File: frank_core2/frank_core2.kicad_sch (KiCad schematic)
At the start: 7 parts

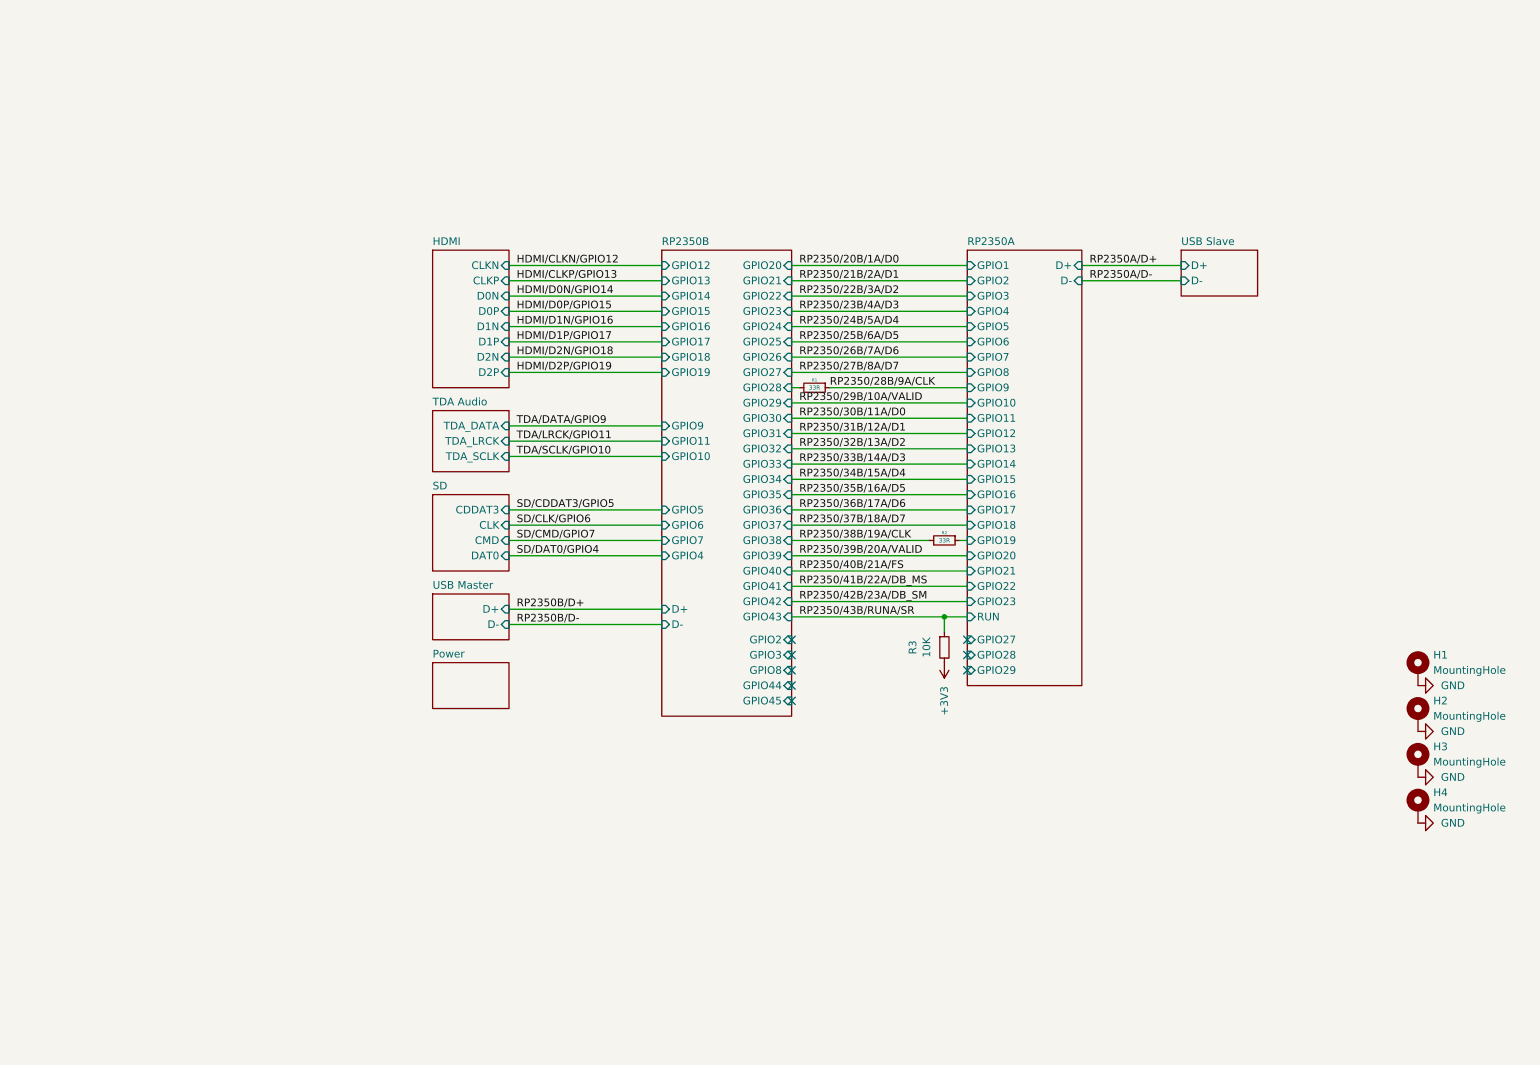
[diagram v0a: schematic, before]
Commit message: Boards WIP
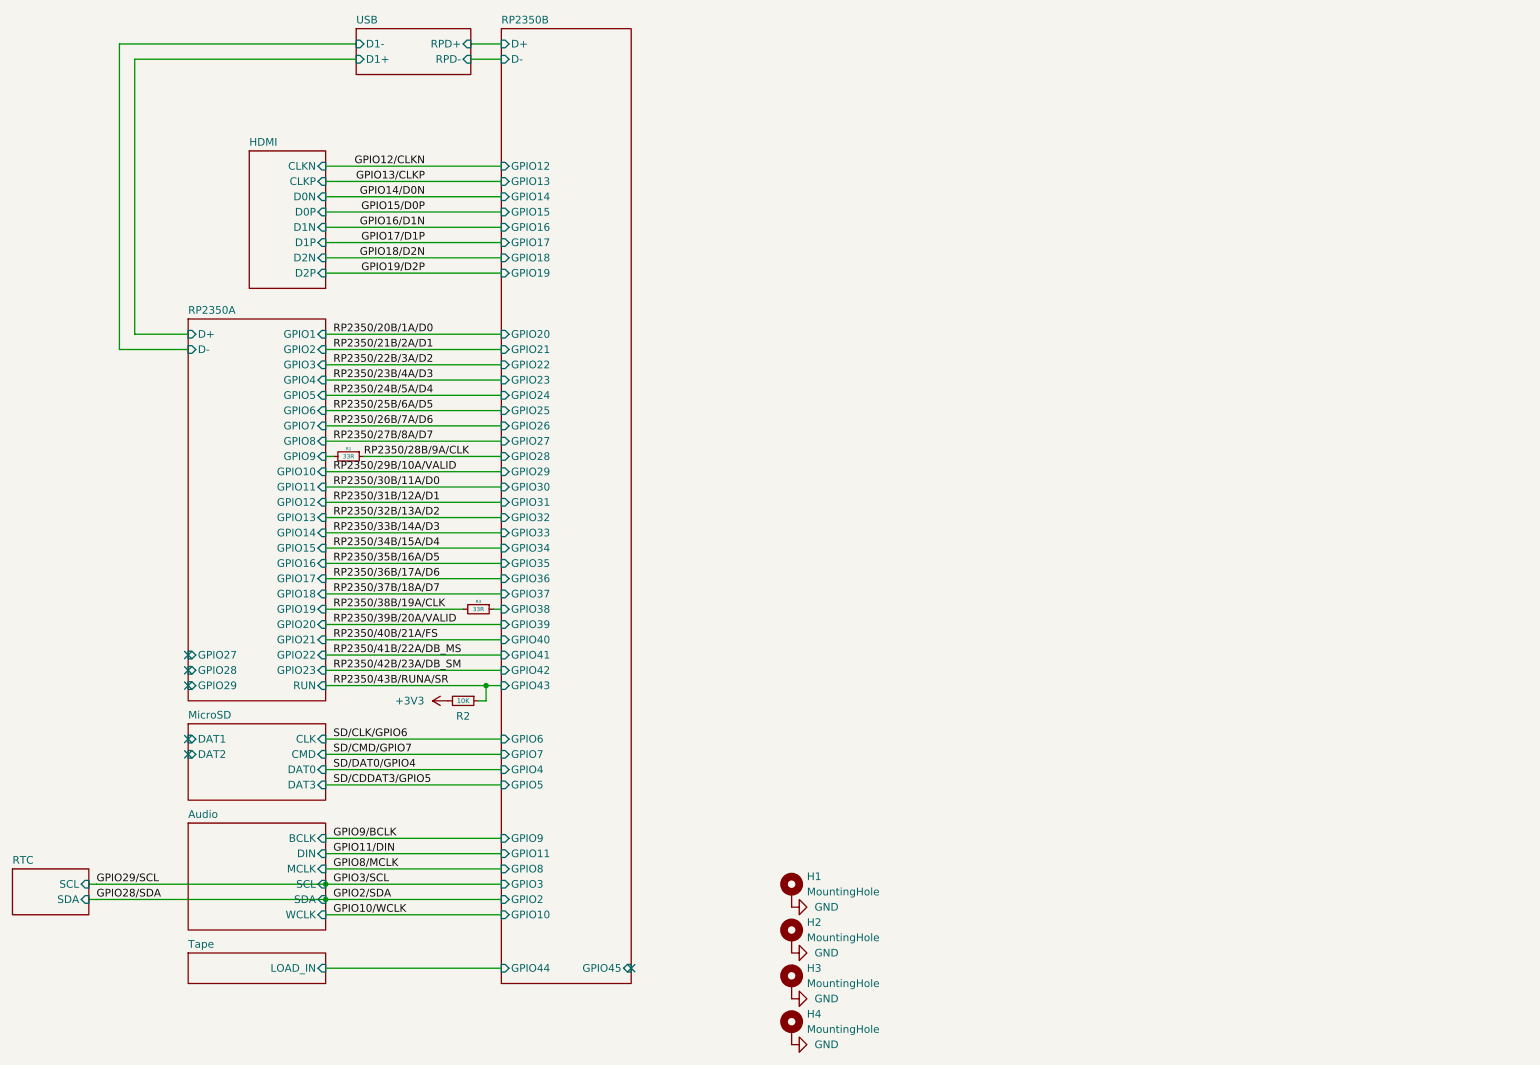
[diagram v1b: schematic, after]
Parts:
- R2: value 33R -> 10K; AliExpress https://www.aliexpress.com/item/1005005945735199.html -> https://www.vishay.com/docs/28952/mcs0402at-mct0603at-mcu08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
- R3: value 10K -> 33R; AliExpress https://www.vishay.com/docs/28952/mcs0402at-mct0603at-mcu08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 -> https://www.aliexpress.com/item/1005005945735199.html
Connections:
- net RP2350A/GPIO19 is gone; now on net RP2350/43B/RUNA/SR: R2.1
- net +3V3: now also R2.2; no longer R3.2
- net RP2350/38B/19A/CLK: now also R3.2; no longer R2.2
- net RP2350/43B/RUNA/SR: no longer R3.1
- net RP2350B/GPIO28 renamed RP2350A/GPIO9
- new net RP2350B/GPIO38: R3.1
- no-connect marks 8 -> 6
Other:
- removed sheet Power
- removed sheet SD
- removed sheet TDA Audio
- removed sheet USB Master
- removed sheet USB Slave
- added sheet Audio (audio.kicad_sch)
- added sheet MicroSD (sd.kicad_sch)
- added sheet RTC (rtc.kicad_sch)
- added sheet Tape (tape.kicad_sch)
- added sheet USB (usb.kicad_sch)
- sheet RP2350B: file rp2350b_master.kicad_sch -> rp2350b.kicad_sch
- moved on the sheet: H1, H2, H3, H4
